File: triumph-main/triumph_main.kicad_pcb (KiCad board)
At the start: 2 copper layers, 99.1 x 86.4 mm, 83 parts, among them J1 JST_XH_vert_01x04, J10 JST_XH_vert_01x04, J2 JST_PH_vert_01x03, J3 JST_PH_vert_01x03, J4 JST_PH_vert_01x06, J5 Conn_BNC, J6 JST_PH_vert_01x03, J7 JST_PH_vert_01x06, J8 JST_PH_vert_01x03, J9 JST_PH_vert_01x03, Q1 J310, U1 LM211P, U2 NE5532AP, U3 NE5532AP, U4 NE5532AP, U5 NE5532AP

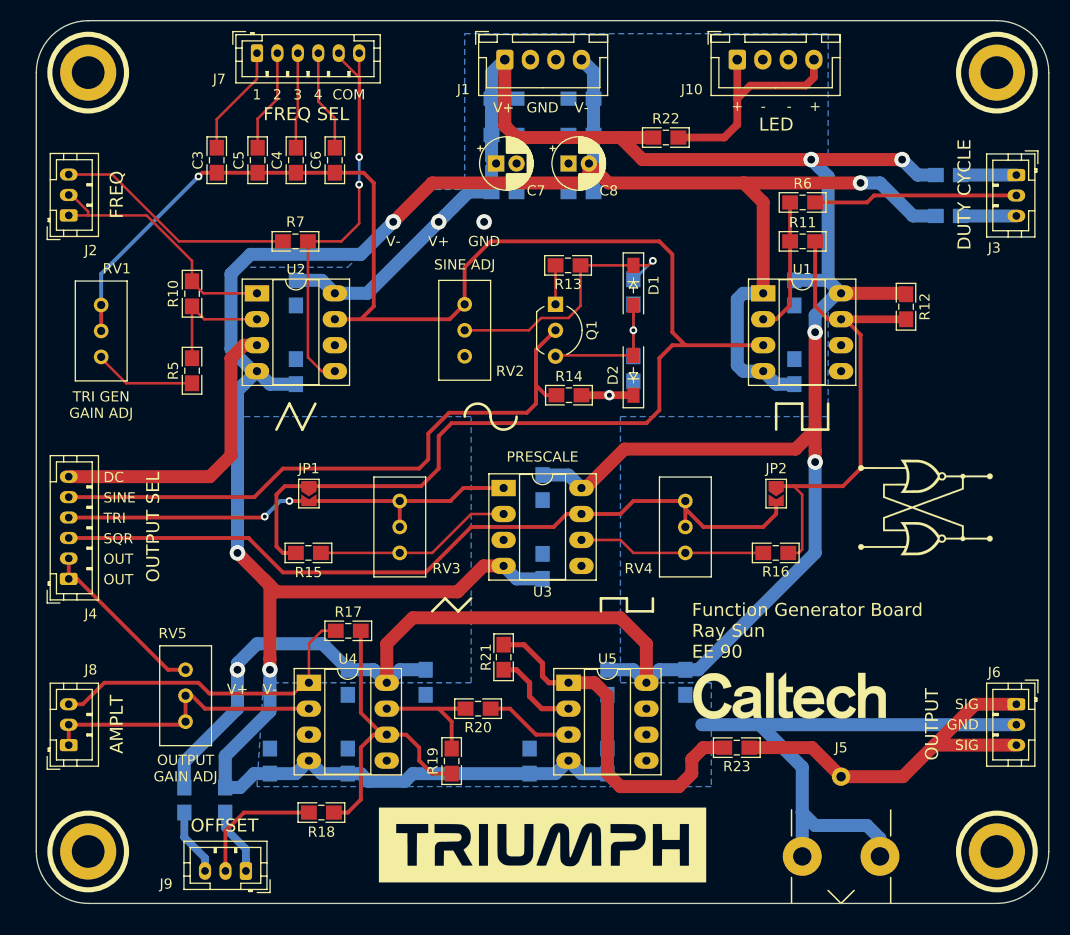
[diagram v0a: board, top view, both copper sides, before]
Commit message: Generate Gerbers
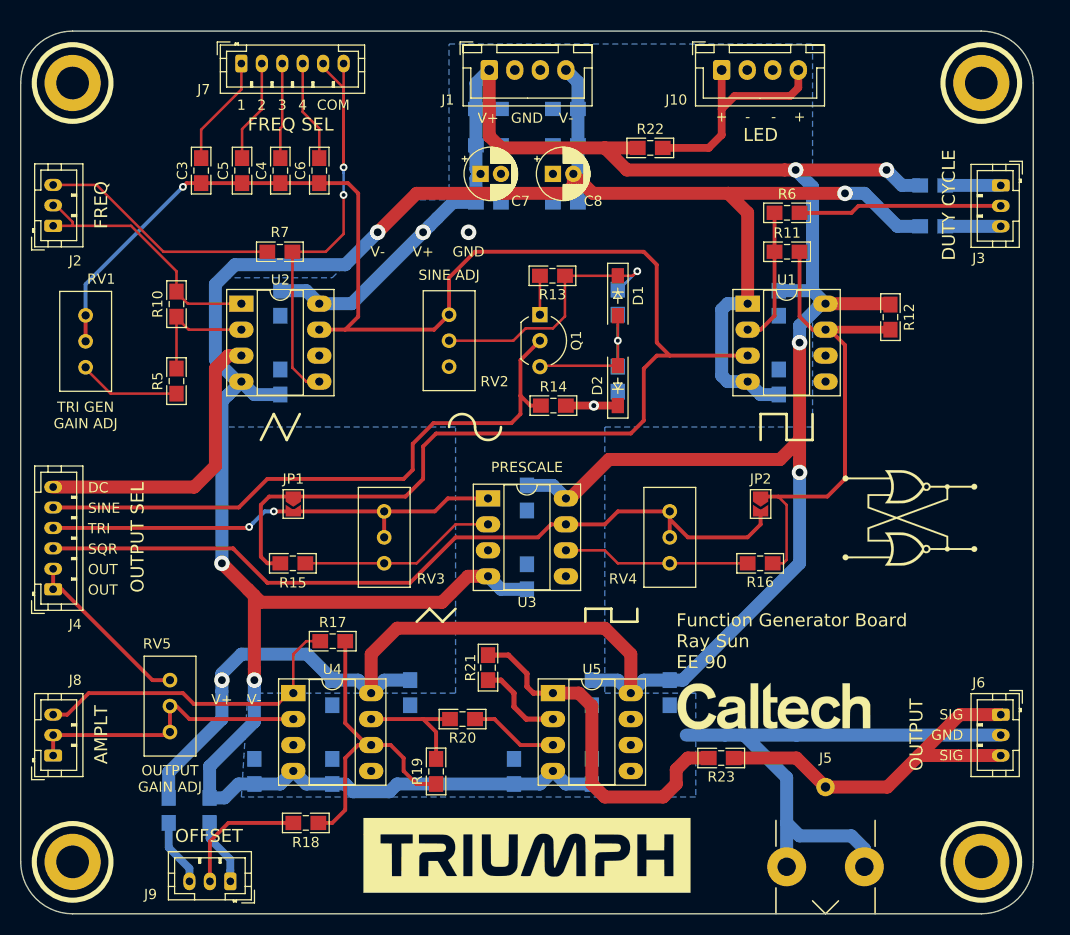
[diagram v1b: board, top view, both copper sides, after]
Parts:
- moved R18 1.83 mm to (122.9, 134.4)
- moved C1 1.83 mm to (169.2, 83.5)
- moved C13 1.83 mm to (140.8, 68.1)
- moved C14 1.83 mm to (148.3, 68.1)
- moved C15 1.83 mm to (140.8, 64.5)
- moved C16 1.83 mm to (148.3, 64.5)
- moved C18 1.83 mm to (144.5, 110.3)
- moved C3 1.83 mm to (112.7, 70.5)
- moved C4 1.83 mm to (120.4, 70.5)
- moved C5 1.83 mm to (116.7, 70.5)
- moved C6 1.83 mm to (124.2, 70.5)
- moved C7 1.83 mm to (140.0, 70.9)
- moved C8 1.83 mm to (147.1, 70.9)
- moved C9 1.83 mm to (120.4, 83.5)
- moved D1 1.83 mm to (153.4, 82.8)
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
